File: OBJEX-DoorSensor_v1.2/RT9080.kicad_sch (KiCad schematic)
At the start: 4 parts, among them U6 RT9080-33GJ5

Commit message: Ready for components placing
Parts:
- U6: footprint KicadLibrary:TSOT-23 -> lib:TSOT-23
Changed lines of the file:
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@@
       (effects (font (size 1.27 1.27)))
     )
-    (property "Footprint" "KicadLibrary:TSOT-23" (at 142.875 76.835 0)
+    (property "Footprint" "lib:TSOT-23" (at 142.875 76.835 0)
       (effects (font (size 1.27 1.27)) hide)
     )

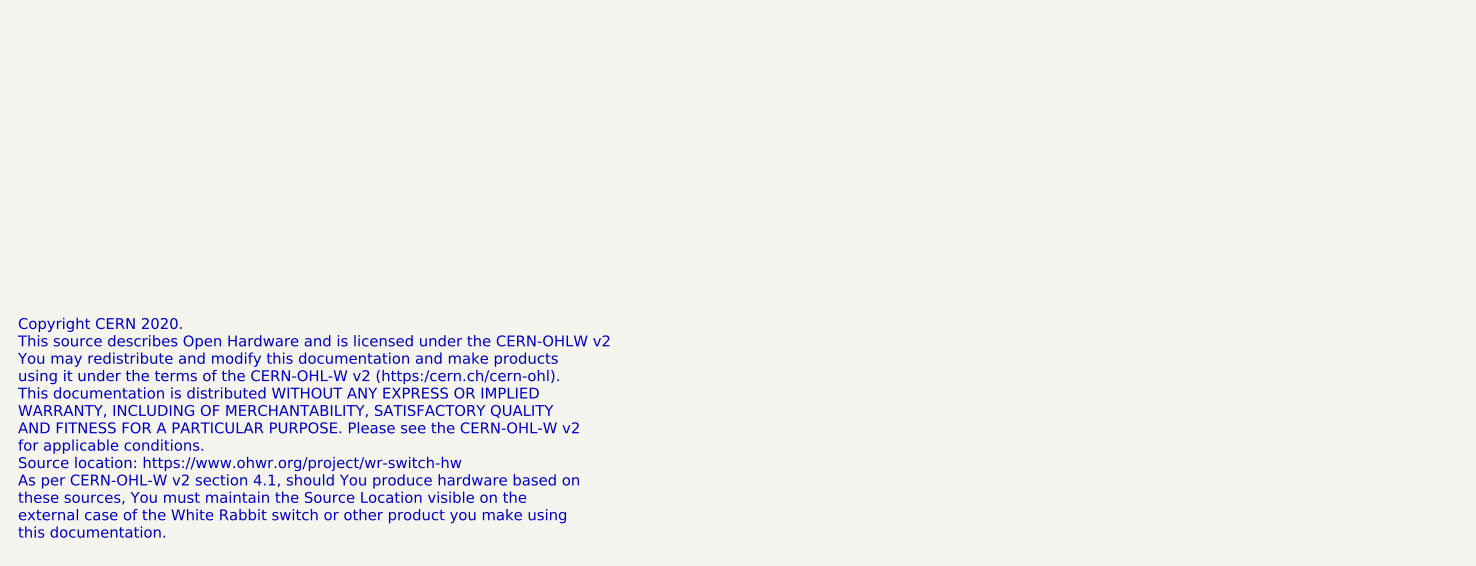
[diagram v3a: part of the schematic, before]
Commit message: update
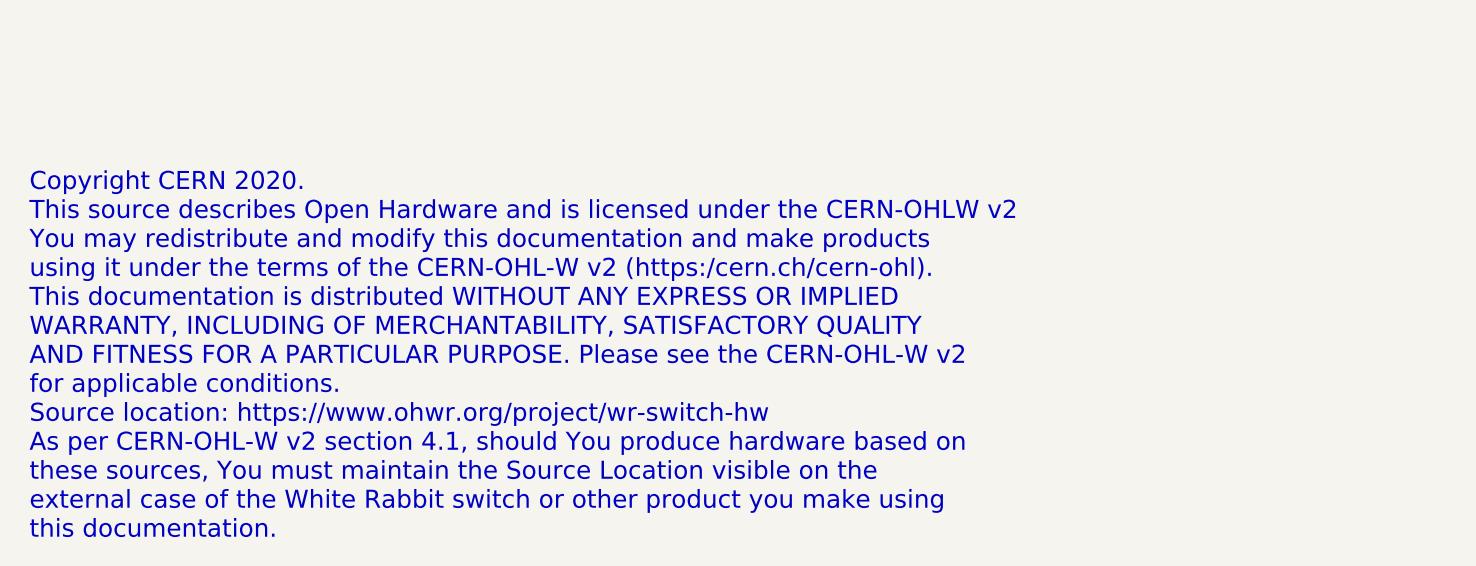
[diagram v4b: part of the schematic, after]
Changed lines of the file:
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@@
   )
   (text "Copyright CERN 2020.\nThis source describes Open Hardware and is licensed under the CERN-OHLW v2\nYou may redistribute and modify this documentation and make products\nusing it under the terms of the CERN-OHL-W v2 (https:/cern.ch/cern-ohl).\nThis documentation is distributed WITHOUT ANY EXPRESS OR IMPLIED\nWARRANTY, INCLUDING OF MERCHANTABILITY, SATISFACTORY QUALITY\nAND FITNESS FOR A PARTICULAR PURPOSE. Please see the CERN-OHL-W v2\nfor applicable conditions.\nSource location: https://www.ohwr.org/project/wr-switch-hw\nAs per CERN-OHL-W v2 section 4.1, should You produce hardware based on\nthese sources, You must maintain the Source Location visible on the\nexternal case of the White Rabbit switch or other product you make using\nthis documentation."
-    (at 16.51 194.31 0)
-    (effects (font (size 1.2 1.2)) (justify left bottom))
+    (at 17.78 194.31 0)
+    (effects (font (size 2 2)) (justify left bottom))
   )
   (symbol (lib_id "power:+3V3") (at 166.751 81.915 270) (unit 1)
